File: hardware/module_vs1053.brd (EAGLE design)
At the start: 109.9 x 68.6 mm, 120 parts, among them IC1 IC_USBLC6-2, IC2 LM1117IMPX-3.3, IC3 PIC32MX795F512, IC4 DP83848, IC5 LM1117MPX-2.5, U1 USD-SOCKETUSD, U3 VS1053-L, X2 CRYSTALS-NOGND-CFPX-217, X3 KUSBVX, Y3 CRYSTAL-GROUNDEDSMD-5X3.2

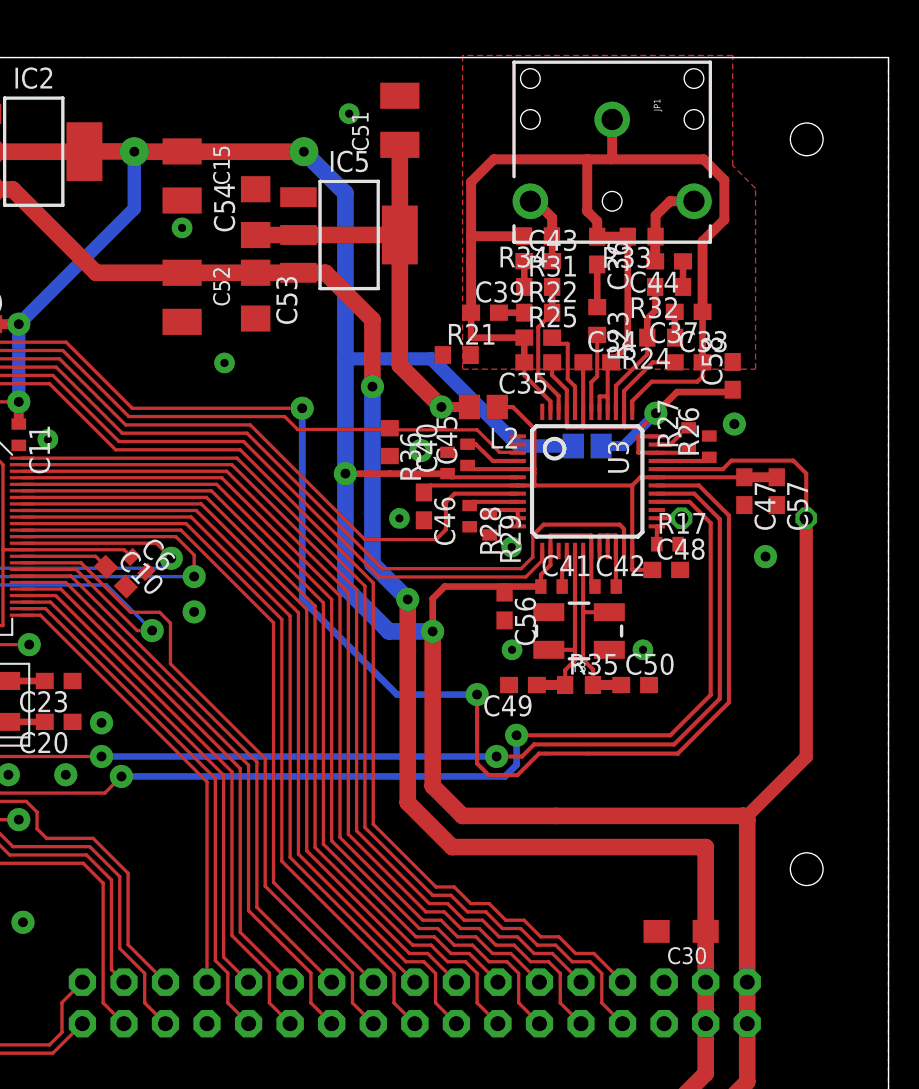
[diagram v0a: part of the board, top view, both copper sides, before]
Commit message: PCB updated
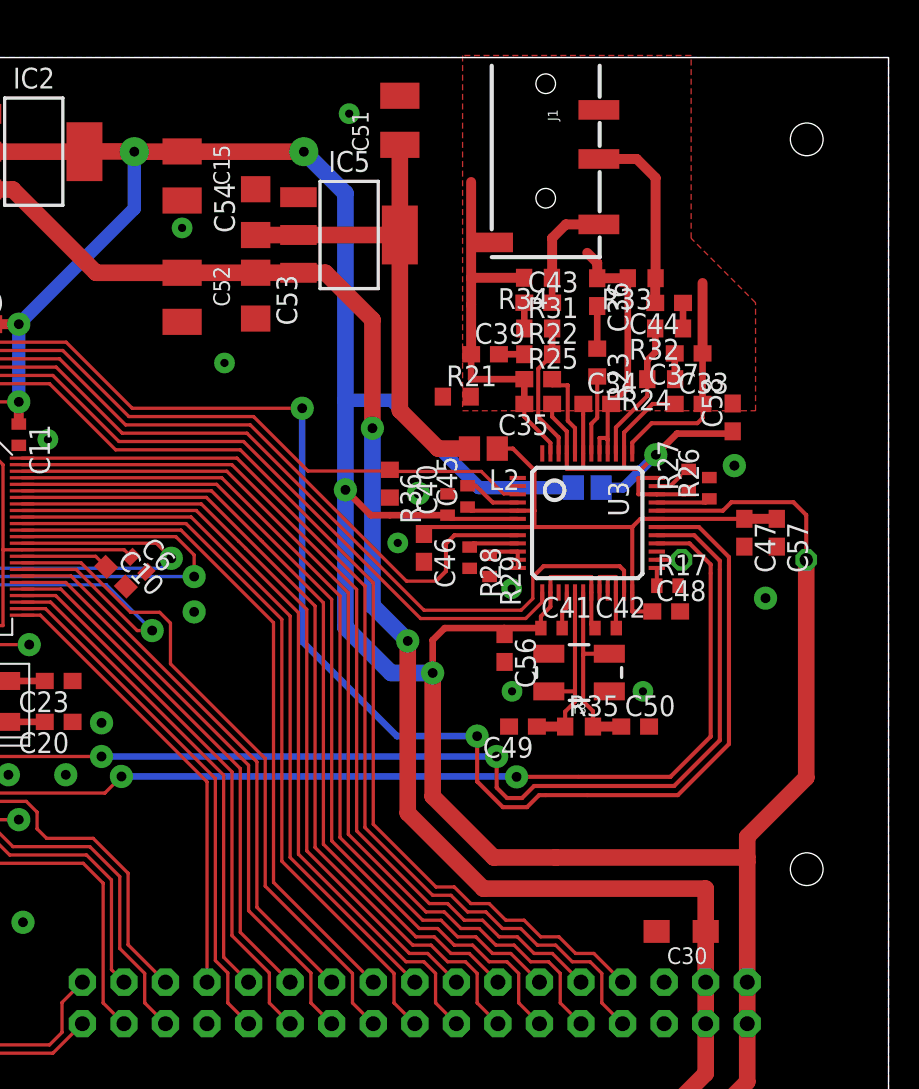
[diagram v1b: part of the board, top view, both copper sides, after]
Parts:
- removed JP1: (no value), SparkFun-Connectors:AUDIO-JACK2
- added J1: AUDIO_JACK_TRRSSMD_RA, SparkFun-Connectors:AUDIO_JACK_3.5MM_TRRS_SMD_RA
- moved C33 2.54 mm to (97.6, 47.4)
- moved C34 2.54 mm to (92.0, 47.4)
- moved C35 2.54 mm to (88.4, 47.4)
- moved C37 2.54 mm to (97.6, 50.5)
- moved C46 2.54 mm to (81.5, 38.6)
- moved C58 2.54 mm to (100.3, 46.6)
- moved L1 2.54 mm to (91.4, 42.3)
- moved R28 2.54 mm to (84.3, 38.0)
- moved C36 2.54 mm to (92.0, 54.2)
- moved C39 2.54 mm to (85.2, 50.4)
- moved C40 2.54 mm to (82.9, 41.3)
- moved C41 2.54 mm to (89.3, 33.7)
- moved C42 2.54 mm to (92.6, 33.7)
- moved C43 2.54 mm to (88.4, 53.6)
- moved C44 2.54 mm to (96.4, 53.6)
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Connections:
- net VS_AGND: now also J1.EARTH; no longer JP1.SLEEVE
- net VS_N$37: now also J1.RING1; no longer JP1.RING
- net VS_N$38: now also J1.TIP; no longer JP1.TIP
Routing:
- net VS_AGND: track 78.1 -> 54.1 mm
- net VS_N$37: track 5.51 -> 11.6 mm
- net VS_N$38: track 4.42 -> 7.17 mm
- net _1V8: track 27.6 -> 30.3 mm, vias 1 -> 0
- net VS_MOSI: track 69.1 -> 71.3 mm
- net VS_SCK: track 71.6 -> 69.5 mm
- net VS_MISO: track 90.8 -> 92.0 mm
- net VBUS: track 191.0 -> 189.9 mm
- net VS_XRST: track 40.9 -> 41.9 mm
- net VS_XDCS: track 43.4 -> 44.5 mm
- net VS_DREQ: track 44.1 -> 45.2 mm
- net VS_XCS: track 51.6 -> 52.6 mm
- net 3V: track 542.6 -> 542.1 mm
